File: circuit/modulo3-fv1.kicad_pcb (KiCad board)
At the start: 2 copper layers, 84 x 52 mm, 57 parts, among them J2 HOLE, J3 CONN_01X03, J4 HOLE, J5 HOLE, J7 HOLE, U1 OPA1642, U10 TLE2426, U2 FV1_CONN, U3 FV-1, U4 PWR_CONN, U5 LM1117 3V3, U6 DIFFAUDIO, U7 AD5142A, U8 AMPCTRL, Y1 32768Hz

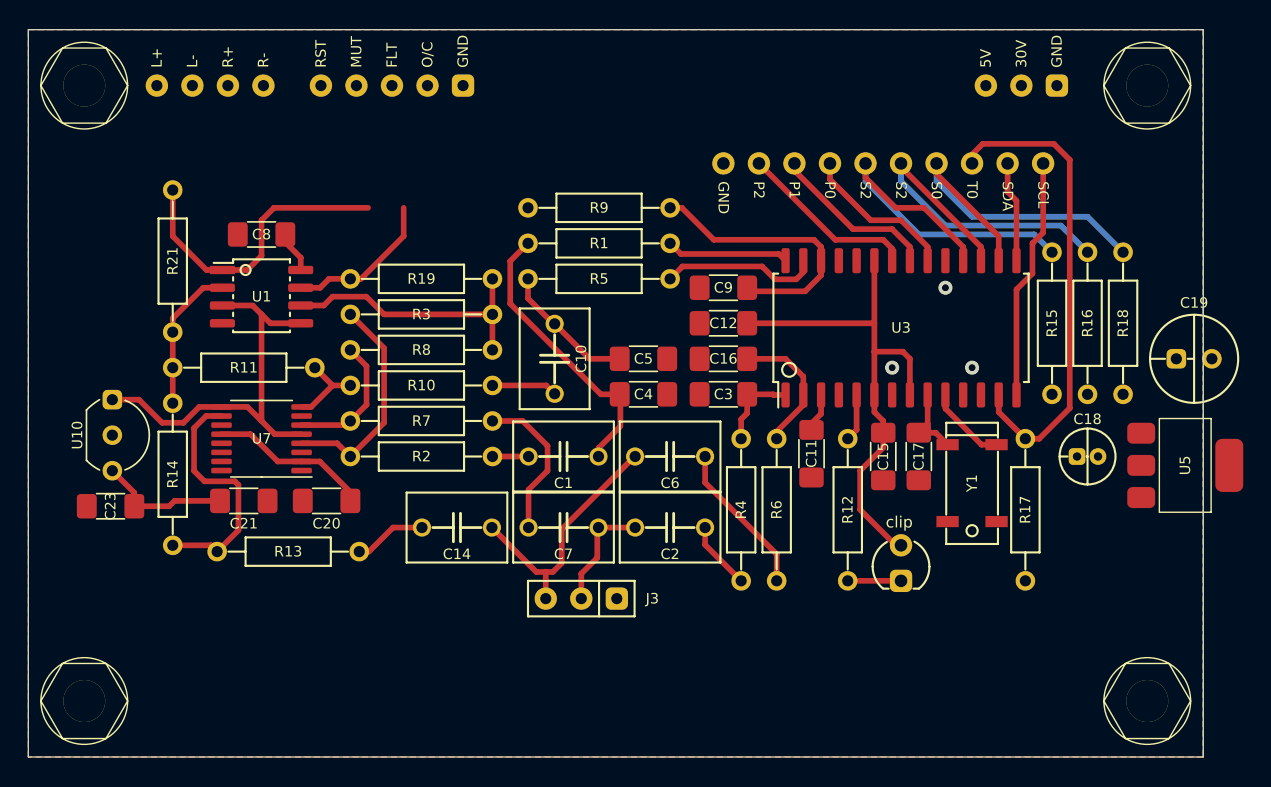
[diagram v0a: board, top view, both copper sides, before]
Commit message: fv-1 mostly done; power progressed
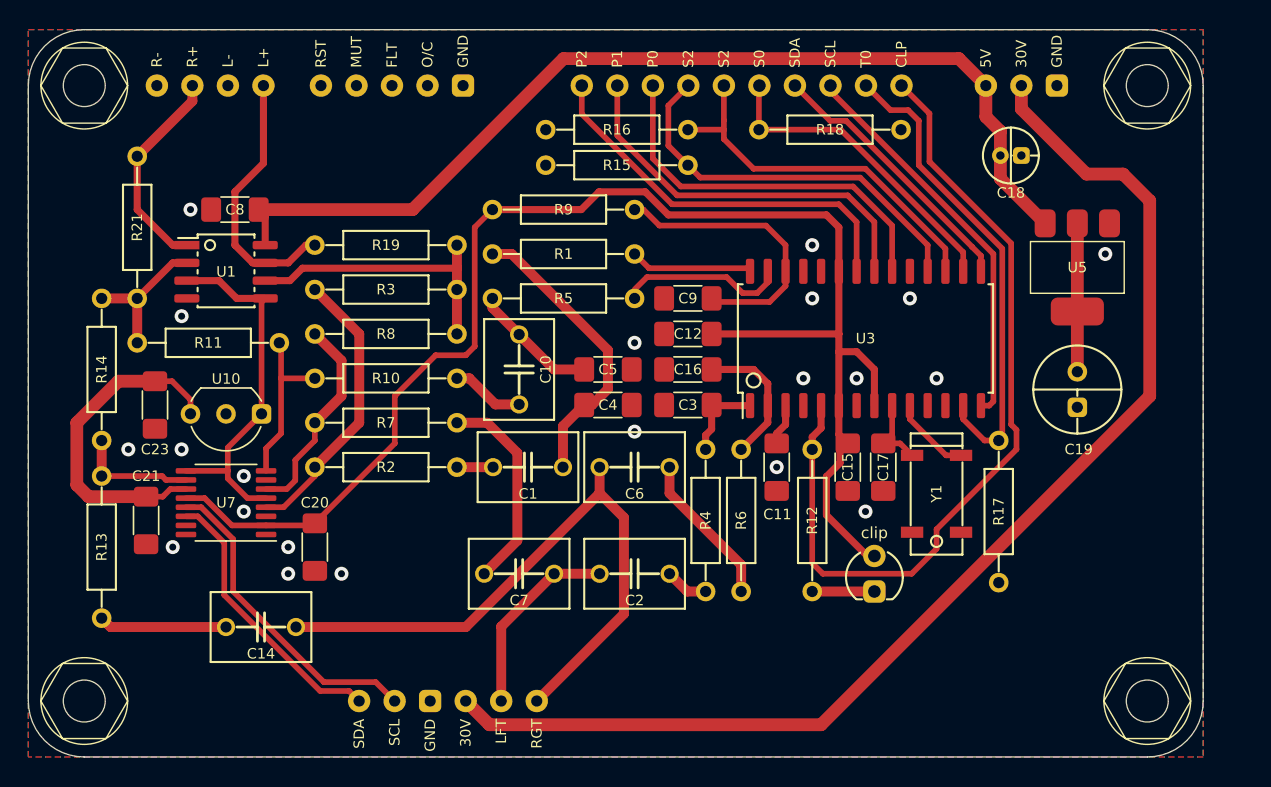
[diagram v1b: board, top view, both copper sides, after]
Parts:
- removed J3: CONN_01X03, myAmp:PIN_1x03
- added U9: PREAMP, myAmp:PREAMP_CONN, F.Cu at (80.0, 98.0)
- moved R16 36.4 mm to (92.1, 57.1), turned to 0 degrees
- moved R15 33.1 mm to (92.1, 59.7), turned to 180 degrees
- moved R18 25.1 mm to (107.3, 57.1), turned to 0 degrees
- moved C18 22.2 mm to (120.2, 59.0), turned to 0 degrees
- moved U5 16.1 mm to (125.0, 67.0), turned to -90 degrees
- moved C14 15.7 mm to (66.6, 92.7)
- moved R13 13.3 mm to (55.2, 87.0), turned to 90 degrees
- moved U2 11.6 mm to (101.0, 54.0), turned to 0 degrees
- moved R14 9.05 mm to (55.2, 74.3)
- moved C19 8.63 mm to (125.0, 75.7), turned to -90 degrees
- moved U10 8.27 mm to (64.1, 77.5), turned to 180 degrees
- moved C23 7.90 mm to (59.1, 76.8), turned to 90 degrees
- moved C21 7.12 mm to (58.4, 85.1), turned to 90 degrees
- moved U7 5.23 mm to (64.1, 83.8)
- moved C7 4.58 mm to (85.1, 88.9)
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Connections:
- R12 pad 2: Net-(R12-Pad2) -> /CLIP
- U2 pad 1: GND -> /POT2
- U2 pad 10: /SCL -> /CLIP
- U2 pad 2: /POT2 -> /POT1
- U2 pad 3: /POT1 -> /POT0
- U2 pad 4: /POT0 -> /S2
- U2 pad 5: /S2 -> /S1
- U2 pad 6: /S1 -> /S0
- U2 pad 7: /S0 -> /FV_SDA
- U2 pad 8: /T0 -> /FV_SCL
- U2 pad 9: /SDA -> /T0
- U3 pad 14: /SCL -> /FV_SCL
- U3 pad 15: /SDA -> /FV_SDA
- U3 pad 5: Net-(R12-Pad2) -> /CLIP
- U4 pad 2: unconnected-(U4-Pad2) -> /30V
- U7 pad 13: /SCL -> SCL
- U7 pad 14: /SDA -> SDA
- U8 pad 1: unconnected-(U8-Pad1) -> GND
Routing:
- net /30V: track 0.00 -> 86.9 mm
- net +5V: track 12.5 -> 95.3 mm
- net +3V3: track 48.7 -> 116.8 mm
- net /CLIP: track 0.00 -> 60.4 mm
- net /FV_SCL: track 0.00 -> 28.4 mm
- net INR: track 18.3 -> 45.7 mm
- net SCL: track 0.00 -> 22.8 mm
- net SDA: track 0.00 -> 20.0 mm
- net /FV_SDA: track 0.00 -> 19.5 mm
- net /SCL: track 17.3 -> 0.00 mm
- net /POT0: track 11.1 -> 27.6 mm
- net /POT1: track 12.0 -> 28.0 mm
- net /POT2: track 12.9 -> 28.4 mm
- net /B2: track 17.7 -> 8.68 mm
- net /OUTL: track 10.9 -> 19.0 mm
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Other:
- outline, holes or cut-outs redrawn

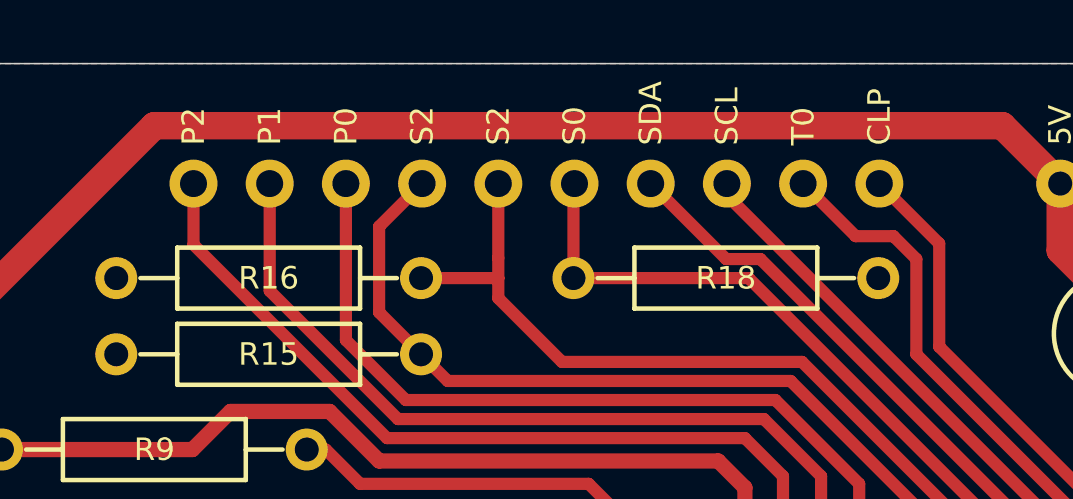
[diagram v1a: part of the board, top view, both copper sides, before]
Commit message: lotsa things :)
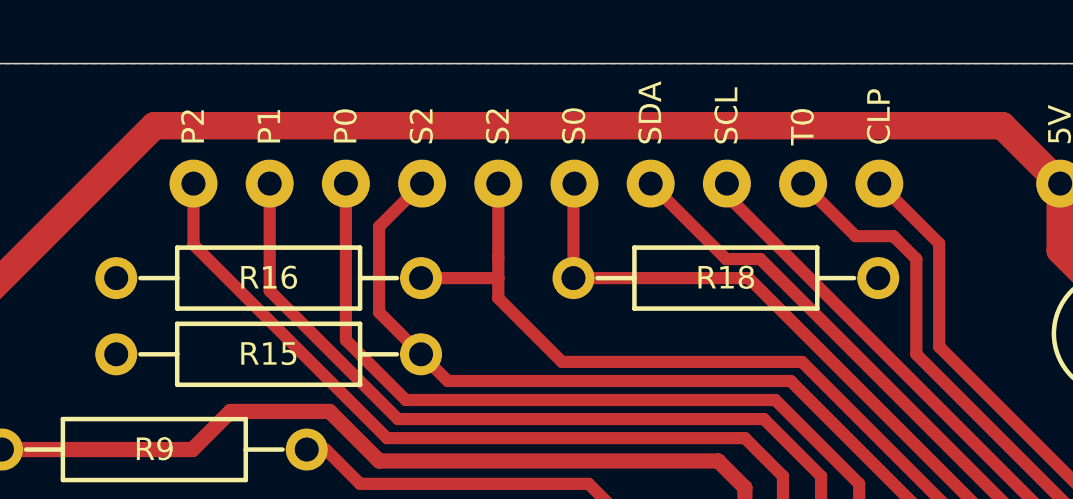
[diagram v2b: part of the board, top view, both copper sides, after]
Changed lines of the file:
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@@
         (effects (font (size 0.75 0.75) (thickness 0.15)))
     )
-    (fp_text user "CLP" (at 11.43 -1.27 90 unlocked) (layer "F.SilkS")
+    (fp_text user "T0" (at 8.89 -1.27 90 unlocked) (layer "F.SilkS")
+        (effects (font (size 0.75 0.75) (thickness 0.15)) (justify left))
+    )
+    (fp_text user "SDA" (at 3.81 -1.27 90 unlocked) (layer "F.SilkS")
+        (effects (font (size 0.75 0.75) (thickness 0.15)) (justify left))
+    )
+    (fp_text user "P1" (at -8.89 -1.27 90 unlocked) (layer "F.SilkS")
         (effects (font (size 0.75 0.75) (thickness 0.15)) (justify left))
     )
     (fp_text user "S0" (at 1.27 -1.27 90 unlocked) (layer "F.SilkS")
-        (effects (font (size 0.75 0.75) (thickness 0.15)) (justify left))
-    )
-    (fp_text user "P0" (at -6.35 -1.27 90 unlocked) (layer "F.SilkS")
         (effects (font (size 0.75 0.75) (thickness 0.15)) (justify left))
     )
@@
         (effects (font (size 0.75 0.75) (thickness 0.15)) (justify left))
     )
-    (fp_text user "P1" (at -8.89 -1.27 90 unlocked) (layer "F.SilkS")
-        (effects (font (size 0.75 0.75) (thickness 0.15)) (justify left))
-    )
-    (fp_text user "T0" (at 8.89 -1.27 90 unlocked) (layer "F.SilkS")
-        (effects (font (size 0.75 0.75) (thickness 0.15)) (justify left))
-    )
-    (fp_text user "SDA" (at 3.81 -1.27 90 unlocked) (layer "F.SilkS")
-        (effects (font (size 0.75 0.75) (thickness 0.15)) (justify left))
-    )
     (fp_text user "S2" (at -3.81 -1.27 90 unlocked) (layer "F.SilkS")
         (effects (font (size 0.75 0.75) (thickness 0.15)) (justify left))
     )
-    (pad "1" thru_hole circle (at -11.43 0) (size 1.6 1.6) (drill 0.9) (layers "*.Cu" "*.Mask")
+    (fp_text user "CLP" (at 11.43 -1.27 90 unlocked) (layer "F.SilkS")
+        (effects (font (size 0.75 0.75) (thickness 0.15)) (justify left))
+    )
+    (fp_text user "P0" (at -6.35 -1.27 90 unlocked) (layer "F.SilkS")
+        (effects (font (size 0.75 0.75) (thickness 0.15)) (justify left))
+    )
+    (pad "1" thru_hole circle (at -11.43 0) (size 1.6 1.6) (drill 0.8) (layers "*.Cu" "*.Mask")
       (net 24 "/POT2") (pinfunction "POT2") (pintype "input"))
-    (pad "2" thru_hole circle (at -8.89 0) (size 1.6 1.6) (drill 0.9) (layers "*.Cu" "*.Mask")
+    (pad "2" thru_hole circle (at -8.89 0) (size 1.6 1.6) (drill 0.8) (layers "*.Cu" "*.Mask")
       (net 23 "/POT1") (pinfunction "POT1") (pintype "input"))
-    (pad "3" thru_hole circle (at -6.35 0) (size 1.6 1.6) (drill 0.9) (layers "*.Cu" "*.Mask")
+    (pad "3" thru_hole circle (at -6.35 0) (size 1.6 1.6) (drill 0.8) (layers "*.Cu" "*.Mask")
       (net 22 "/POT0") (pinfunction "POT0") (pintype "input"))
-    (pad "4" thru_hole circle (at -3.81 0) (size 1.6 1.6) (drill 0.9) (layers "*.Cu" "*.Mask")
+    (pad "4" thru_hole circle (at -3.81 0) (size 1.6 1.6) (drill 0.8) (layers "*.Cu" "*.Mask")
       (net 27 "/S2") (pinfunction "S2") (pintype "input"))
-    (pad "5" thru_hole circle (at -1.27 0) (size 1.6 1.6) (drill 0.9) (layers "*.Cu" "*.Mask")
+    (pad "5" thru_hole circle (at -1.27 0) (size 1.6 1.6) (drill 0.8) (layers "*.Cu" "*.Mask")
       (net 26 "/S1") (pinfunction "S1") (pintype "input"))
-    (pad "6" thru_hole circle (at 1.27 0) (size 1.6 1.6) (drill 0.9) (layers "*.Cu" "*.Mask")
+    (pad "6" thru_hole circle (at 1.27 0) (size 1.6 1.6) (drill 0.8) (layers "*.Cu" "*.Mask")
       (net 25 "/S0") (pinfunction "S0") (pintype "input"))
-    (pad "7" thru_hole circle (at 3.81 0) (size 1.6 1.6) (drill 0.9) (layers "*.Cu" "*.Mask")
+    (pad "7" thru_hole circle (at 3.81 0) (size 1.6 1.6) (drill 0.8) (layers "*.Cu" "*.Mask")
       (net 29 "/FV_SDA") (pinfunction "SDA") (pintype "input"))
-    (pad "8" thru_hole circle (at 6.35 0) (size 1.6 1.6) (drill 0.9) (layers "*.Cu" "*.Mask")
+    (pad "8" thru_hole circle (at 6.35 0) (size 1.6 1.6) (drill 0.8) (layers "*.Cu" "*.Mask")
       (net 30 "/FV_SCL") (pinfunction "SCL") (pintype "input"))
-    (pad "9" thru_hole circle (at 8.89 0) (size 1.6 1.6) (drill 0.9) (layers "*.Cu" "*.Mask")
+    (pad "9" thru_hole circle (at 8.89 0) (size 1.6 1.6) (drill 0.8) (layers "*.Cu" "*.Mask")
       (net 28 "/T0") (pinfunction "T0") (pintype "input"))
-    (pad "10" thru_hole circle (at 11.43 0) (size 1.6 1.6) (drill 0.9) (layers "*.Cu" "*.Mask")
+    (pad "10" thru_hole circle (at 11.43 0) (size 1.6 1.6) (drill 0.8) (layers "*.Cu" "*.Mask")
       (net 42 "/CLIP") (pinfunction "CLP") (pintype "input"))
     (model "${KIPRJMOD}/myAmp.pretty/models/PinHeader_1x10_P2.54mm_Vertical.step"
